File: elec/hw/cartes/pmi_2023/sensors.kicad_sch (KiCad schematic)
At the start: 50 parts, among them SW1 SPVT210104, SW2 SPVT110106, SW3 SPVT110106, SW4 SPVT210104, U10 tof_sensor_master, U11 tof_sensor_master, U12 LSM6DSO32XTR, U13 GP2S60B, U14 GP2S60B, U15 GP2S60B, U16 GP2S60B, U17 tof_sensor_master, U18 tof_sensor_master, U19 GP2S60B, U20 GP2S60B, U21 tof_sensor_master, U22 tof_sensor_master, U5 AD8531ARTZ, U6 tof_sensor_master, U7 tof_sensor_master, U8 GP2S60B, U9 GP2S60B

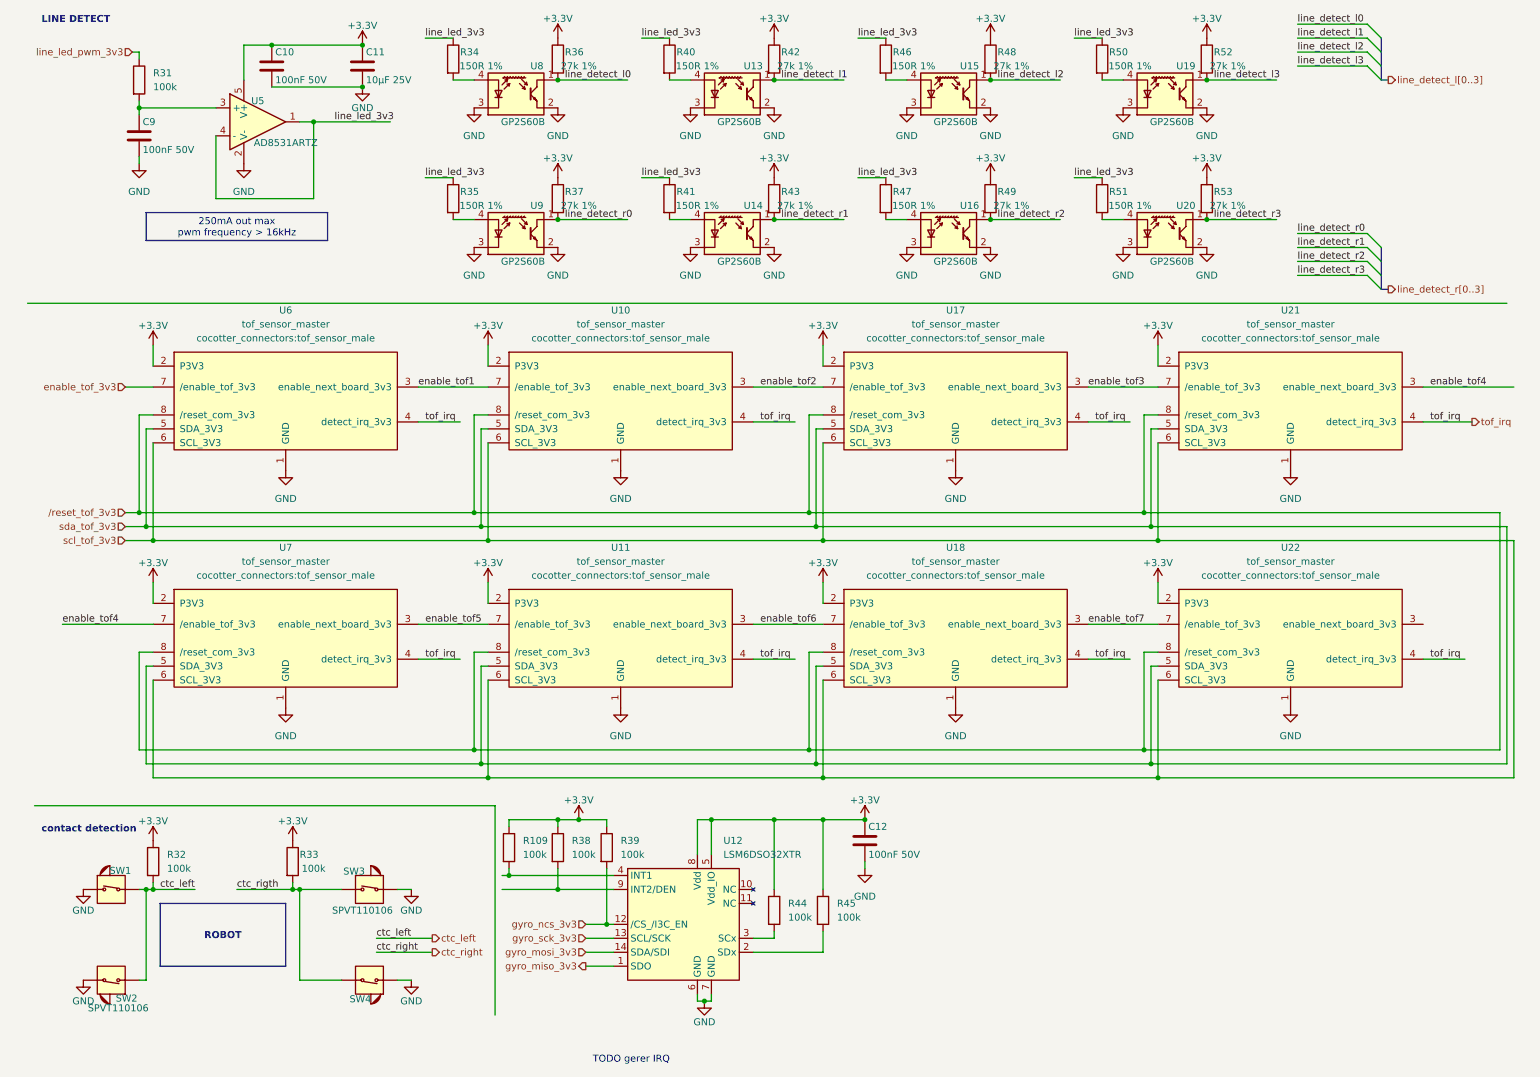
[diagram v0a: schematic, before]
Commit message: wip
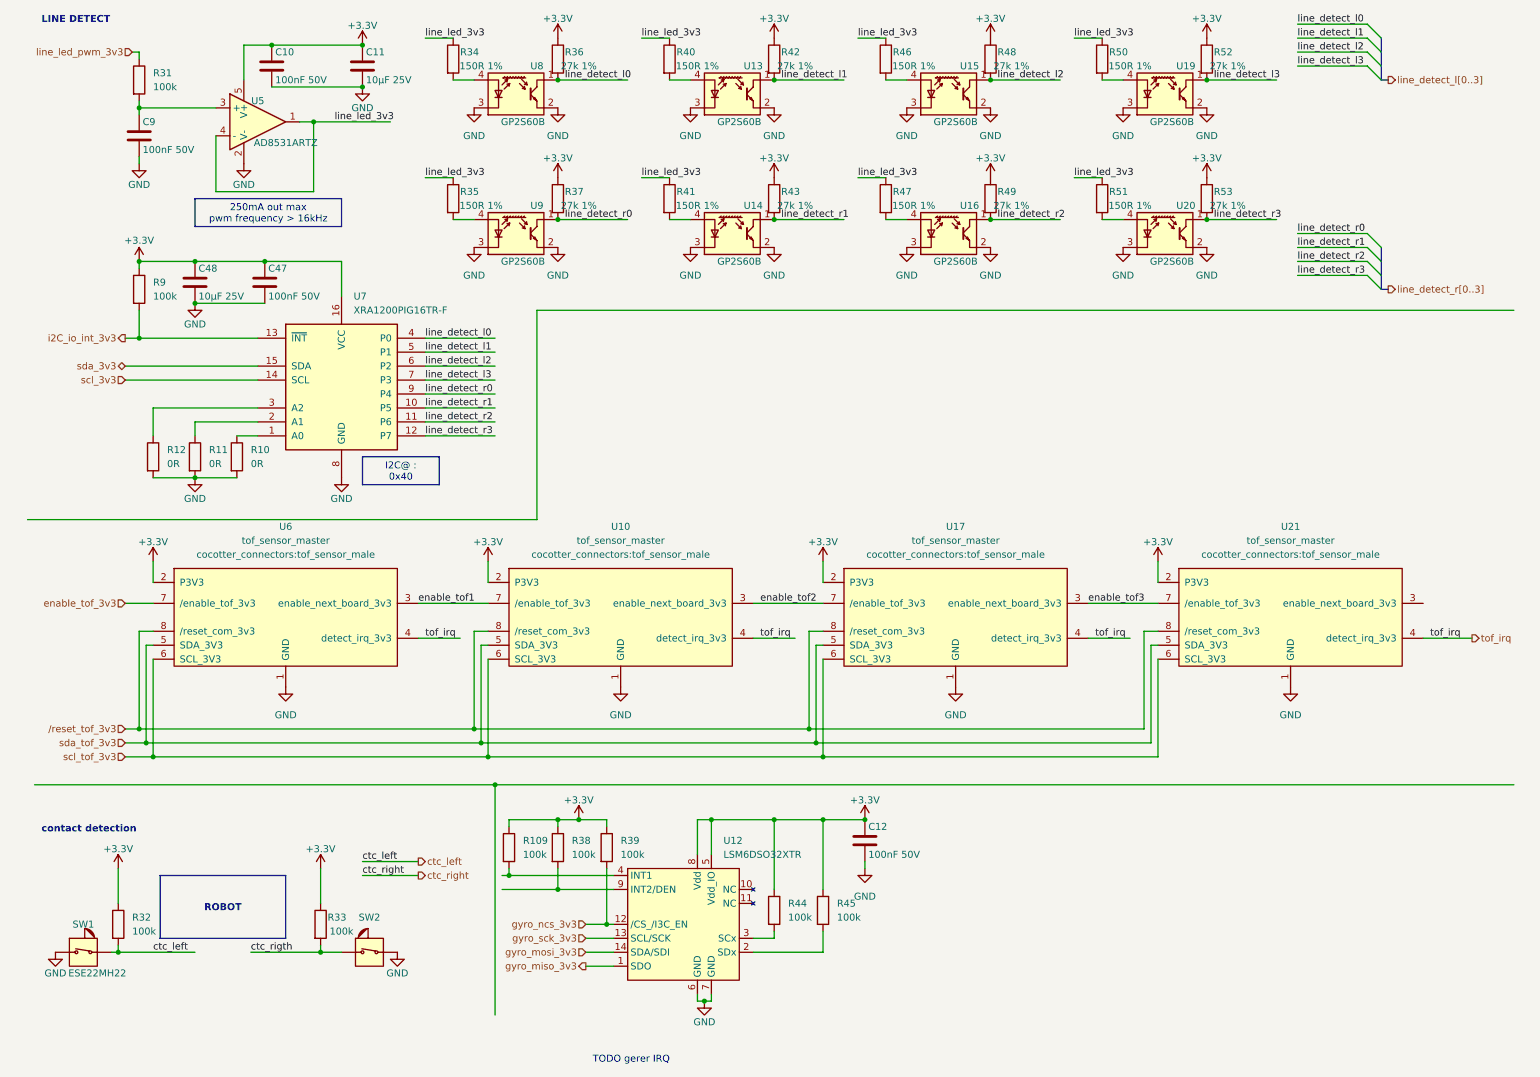
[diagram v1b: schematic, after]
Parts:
- removed SW1, SW4: SPVT210104, symbol cocotter_connectors:SPVT210104
- removed SW2, SW3: SPVT110106, symbol cocotter_connectors:SPVT110106
- removed U11, U18, U22, U7: tof_sensor_master, cocotter_connectors:tof_sensor_male, symbol cocotter_connectors:tof_sensor_master
- added C47: 100nF 50V, cocotter_capacitors:C_0603_1608Metric, symbol cocotter_capacitors:C_100nF_50V_0603
- added C48: 10µF 25V, cocotter_capacitors:C_0805_2012Metric, symbol cocotter_capacitors:C_10µF_16V_0805_X5R
- added R10, R11, R12: 0R, cocotter_resistor:r0603_reflow, symbol cocotter_resistors:R_0R_0603
- added R9: 100k, cocotter_resistor:r0603_reflow, symbol cocotter_resistors:R_100k_0603_1%
- added SW1: ESE22MH22, cocotter_connectors:ESE22MH22, symbol cocotter_connectors:ESE22MH22
- added SW2: ESE22MH24, cocotter_connectors:ESE22MH24, symbol cocotter_connectors:ESE22MH24
- added U7: XRA1200PIG16TR-F, cocotter_ic:TSSOP-16_4.4x5mm_P0.65mm, symbol cocotter_ic:XRA1200PIG16TR-F
- U5: footprint cocotter_ic:SOT23-5 -> cocotter_ic:SOT-23-5
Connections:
- net +3.3V: now also C47.1, C48.1, R9.1, U7.16 (VCC)
- net GND: now also C47.2, C48.2, R10.2, R11.2, R12.2, SW1.1, SW2.2, U7.8 (GND)
- net ctc_left: now also SW1.2
- net ctc_rigth: now also SW2.1
- net line_detect_l0: now also U7.4 (P0)
- net line_detect_l1: now also U7.5 (P1)
- net line_detect_l2: now also U7.6 (P2)
- net line_detect_l3: now also U7.7 (P3)
- net line_detect_r0: now also U7.9 (P4)
- net line_detect_r1: now also U7.10 (P5)
- net line_detect_r2: now also U7.11 (P6)
- net line_detect_r3: now also U7.12 (P7)
- net enable_tof4: no longer names the net of U21.3 (enable_next_board_3v3)
- new net: R12.1, U7.3 (A2)
- new net: R10.1, U7.1 (A0)
- new net: R11.1, U7.2 (A1)
- new net i2C_io_int_3v3: R9.2, U7.13 (~{INT})
- new net scl_3v3: U7.14 (SCL)
- new net sda_3v3: U7.15 (SDA)
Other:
- moved on the sheet: R32, R33, U10, U17, U21, U6
